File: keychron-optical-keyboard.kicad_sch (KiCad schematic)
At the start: 223 parts

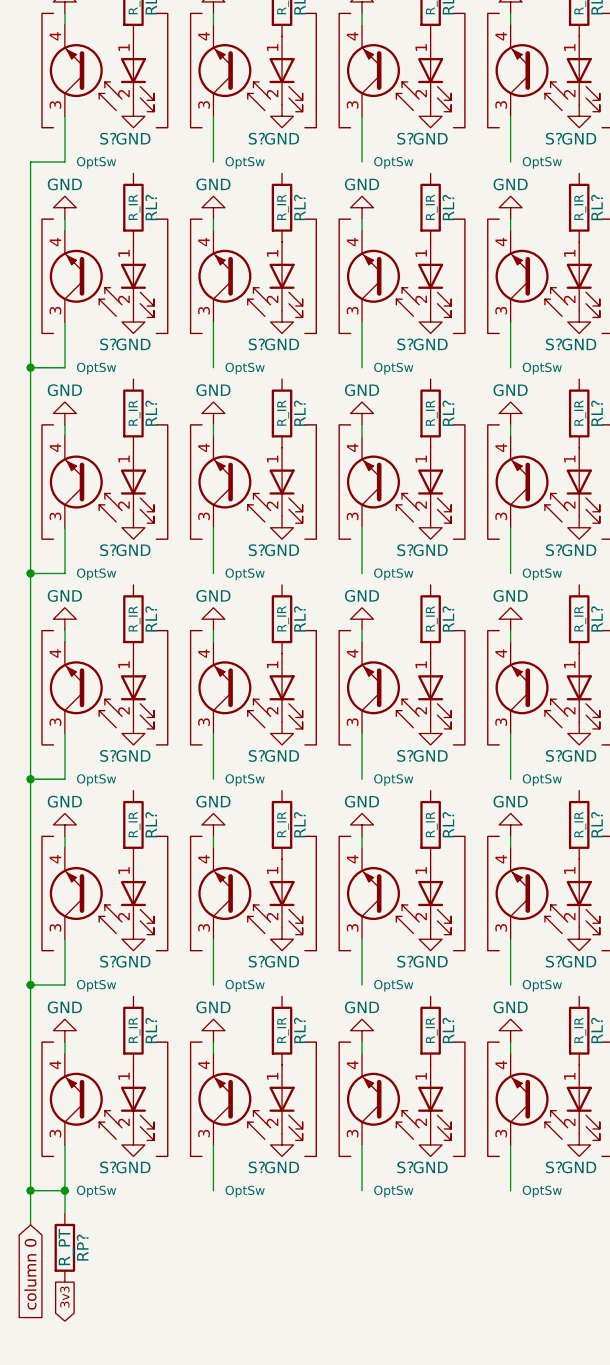
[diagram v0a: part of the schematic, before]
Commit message: added readme
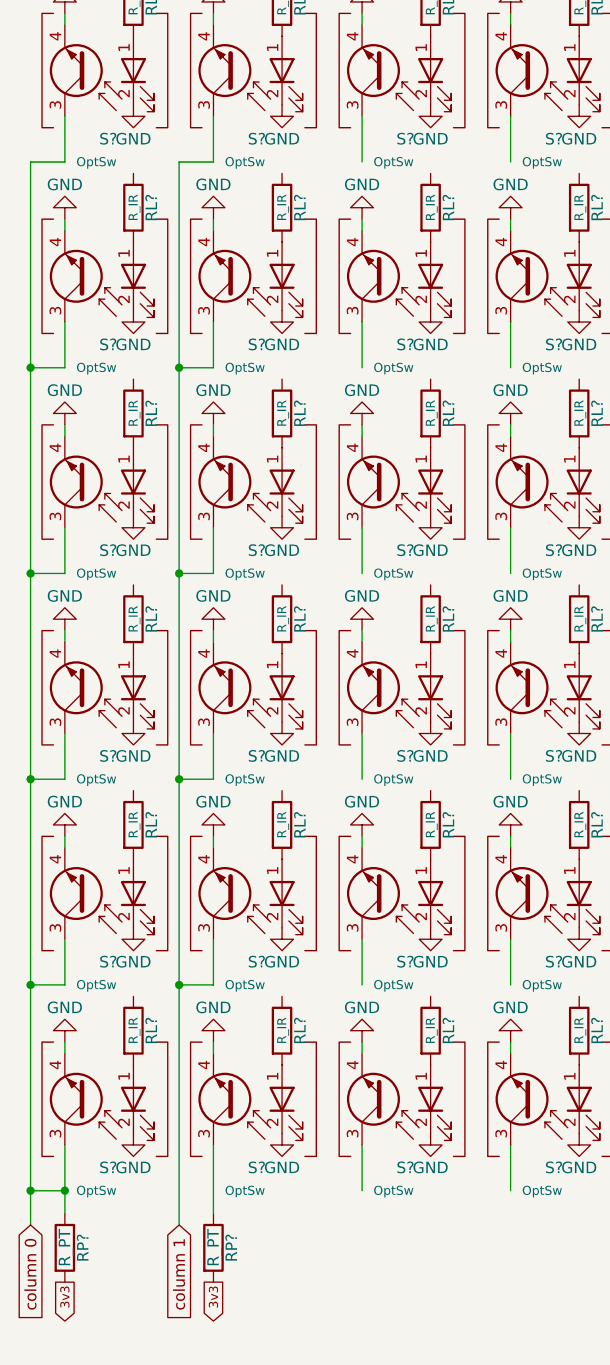
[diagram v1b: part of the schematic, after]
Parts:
- added RP?: R_PT, Resistor_SMD:R_0805_2012Metric_Pad1.20x1.40mm_HandSolder, symbol MySymbols:R_PT
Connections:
- net 3v3: now also RP?.2
- net at S?.3 (C): now also RP?.1
- net column 1: now reaches S?.3 (C)
- net column 1: now also S?.3 (C), S?.3 (C), S?.3 (C), S?.3 (C)
